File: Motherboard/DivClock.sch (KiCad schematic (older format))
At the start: 15 parts, among them SW1 TURBO, SW2 FREEZE, U15 74LS257, U5 ATF750LVC, U9 40106, Y1 14.31818 MHz, Y2 24.000 MHz

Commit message: Large sync
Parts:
- U5: symbol fdc:ATF750LVC -> Motherboard-rescue:ATF750LVC-fdc
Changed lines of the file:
@@
 $Descr A4 11693 8268
 encoding utf-8
-Sheet 3 8
+Sheet 3 10
 Title ""
 Date ""
@@
 	4900 3625 4900 4200
 $Comp
-L fdc:ATF750LVC U5
+L Motherboard-rescue:ATF750LVC-fdc U5
 U 1 1 5C531418
 P 8700 3025

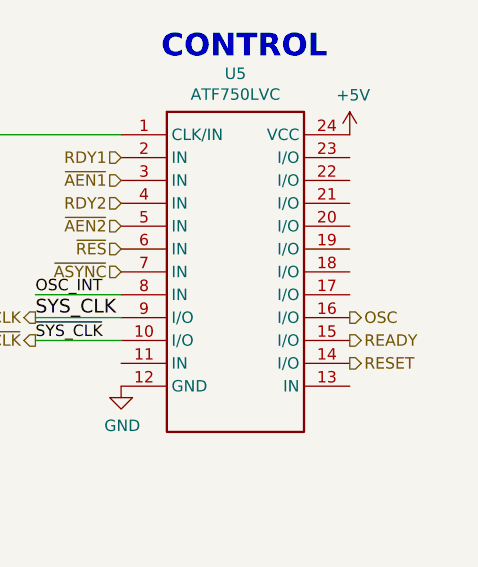
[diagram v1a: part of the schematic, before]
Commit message: LARGE sync
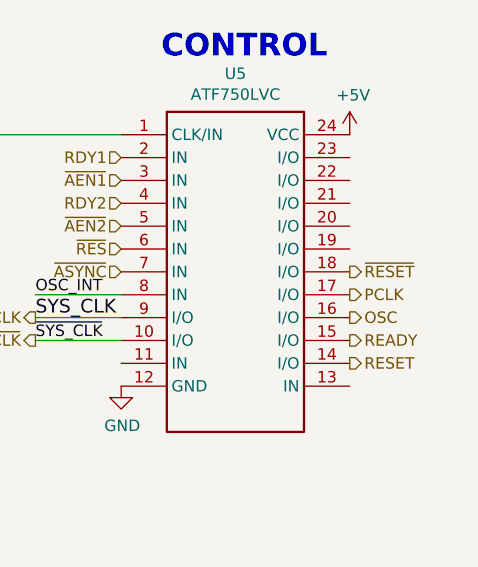
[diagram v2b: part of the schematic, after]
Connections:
- net PCLK: now reaches U5.17 (I/O)
- net ~RESET: now reaches U5.18 (I/O)
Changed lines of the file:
@@
 EESchema Schematic File Version 4
 LIBS:Motherboard-cache
-EELAYER 26 0
+EELAYER 29 0
 EELAYER END
 $Descr A4 11693 8268
@@
 Wire Wire Line
 	3975 1450 4275 1450
+Text HLabel 9200 3125 2    50   Output ~ 0
+PCLK
+Text HLabel 9200 3025 2    50   Output ~ 0
+~RESET
 $EndSCHEMATC
